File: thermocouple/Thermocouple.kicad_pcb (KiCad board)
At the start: 2 copper layers, 50 x 50 mm, 39 parts, among them IC301 nPM1300-QEXX, IC701 MCP9600, M701 BM15C, SW701 Join, X301 Charge, X302 Battery, X701 Debug, X702 Thermocouple

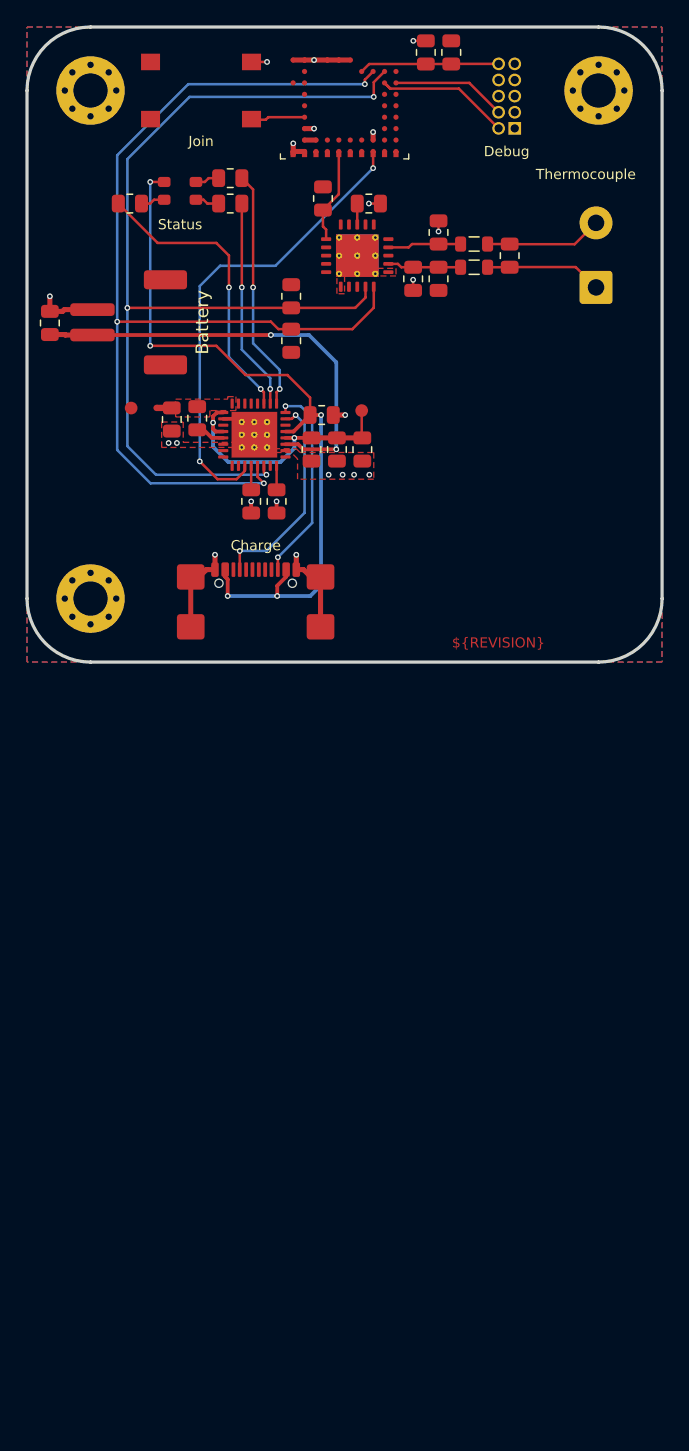
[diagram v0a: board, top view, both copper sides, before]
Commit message: Prepare release 1.0.0
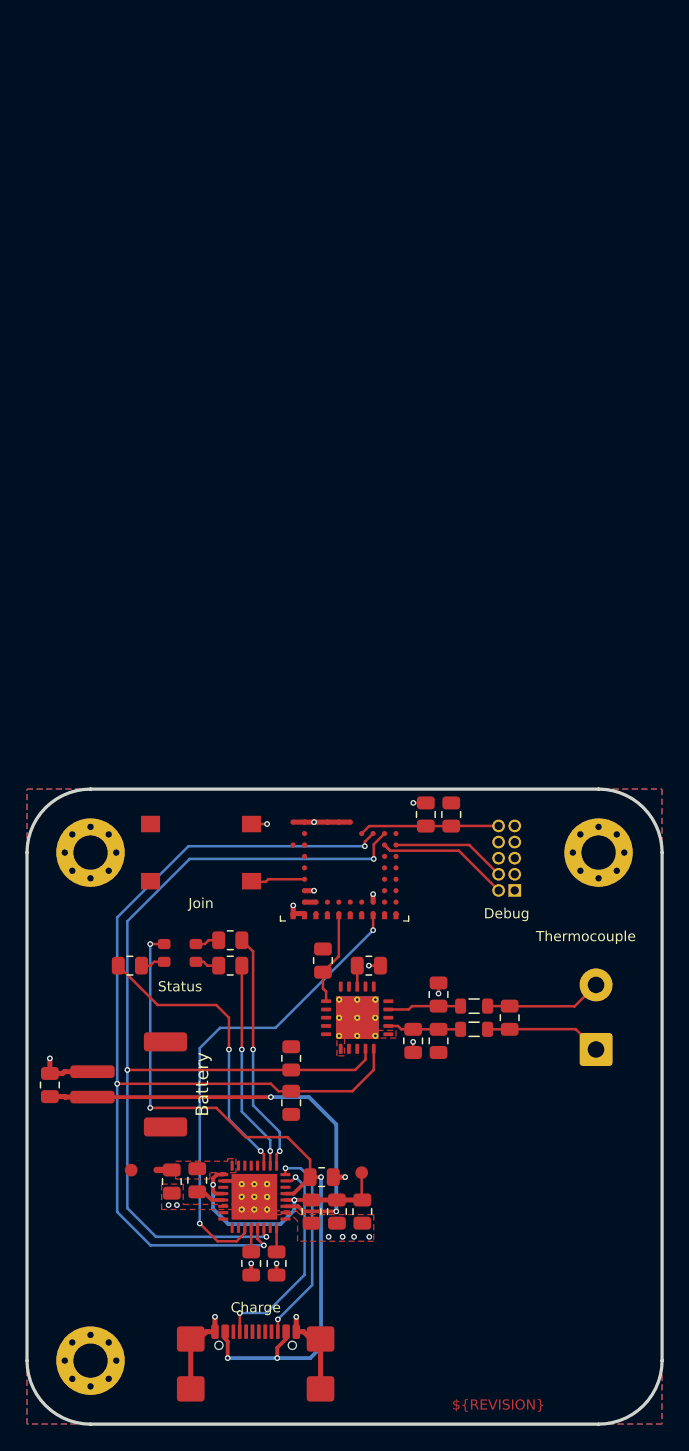
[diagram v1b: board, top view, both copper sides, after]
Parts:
- moved C301 60.0 mm to (199.2, 160.6)
- moved C303 60.0 mm to (177.8, 153.3)
- moved L301 60.0 mm to (189.4, 160.8)
- moved NT301 60.0 mm to (186.7, 160.0)
- moved R706 60.0 mm to (208.4, 146.2)
- moved C302 60.0 mm to (193.7, 167.3)
- moved C305 60.0 mm to (187.4, 160.9)
- moved C701 60.0 mm to (207.4, 132.0)
- moved C703 60.0 mm to (202.9, 143.9)
- moved C704 60.0 mm to (214.0, 148.0)
- moved D401 60.0 mm to (188.1, 142.9)
- moved FB701 60.0 mm to (211.2, 148.9)
- moved FB702 60.0 mm to (211.2, 147.1)
- moved IC301 60.0 mm to (193.9, 162.1)
- moved IC701 60.0 mm to (202.0, 148.0)
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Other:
- board text removed: "Impedance Table"

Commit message: Update outputs (release)
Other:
- board text added: "1.492mm"
- board text removed: "0.196mm"
- board text removed: "1.03mm"
- board text removed: "Inner1 (GND)"
- board text removed: "Inner2"
- board text removed: "Plane"
- board text removed: "Prepreg"
